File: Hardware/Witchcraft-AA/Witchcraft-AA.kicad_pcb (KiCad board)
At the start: 2 copper layers, 180 x 81 mm, 20 parts, among them J0 USB_C_Molex_201267-0005, J1 USB_C_Molex_201267-0005, J2 TE_2129567-1, U1 Z1 extreme, U2 LM26420-Q1xx-xxxx

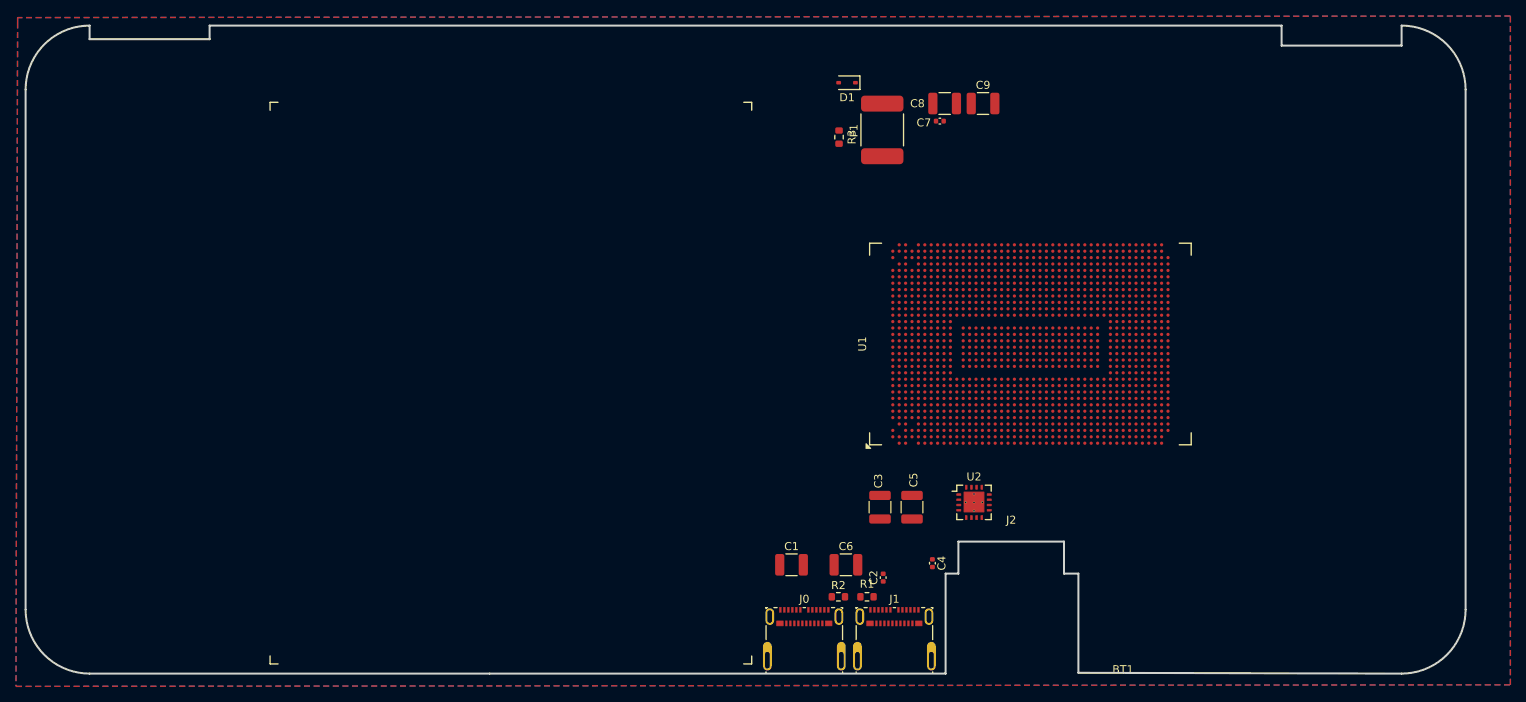
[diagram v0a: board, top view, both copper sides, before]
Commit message: Some chances to start/rectangle-buttons in mech, and startedmaking the M.2 ports.
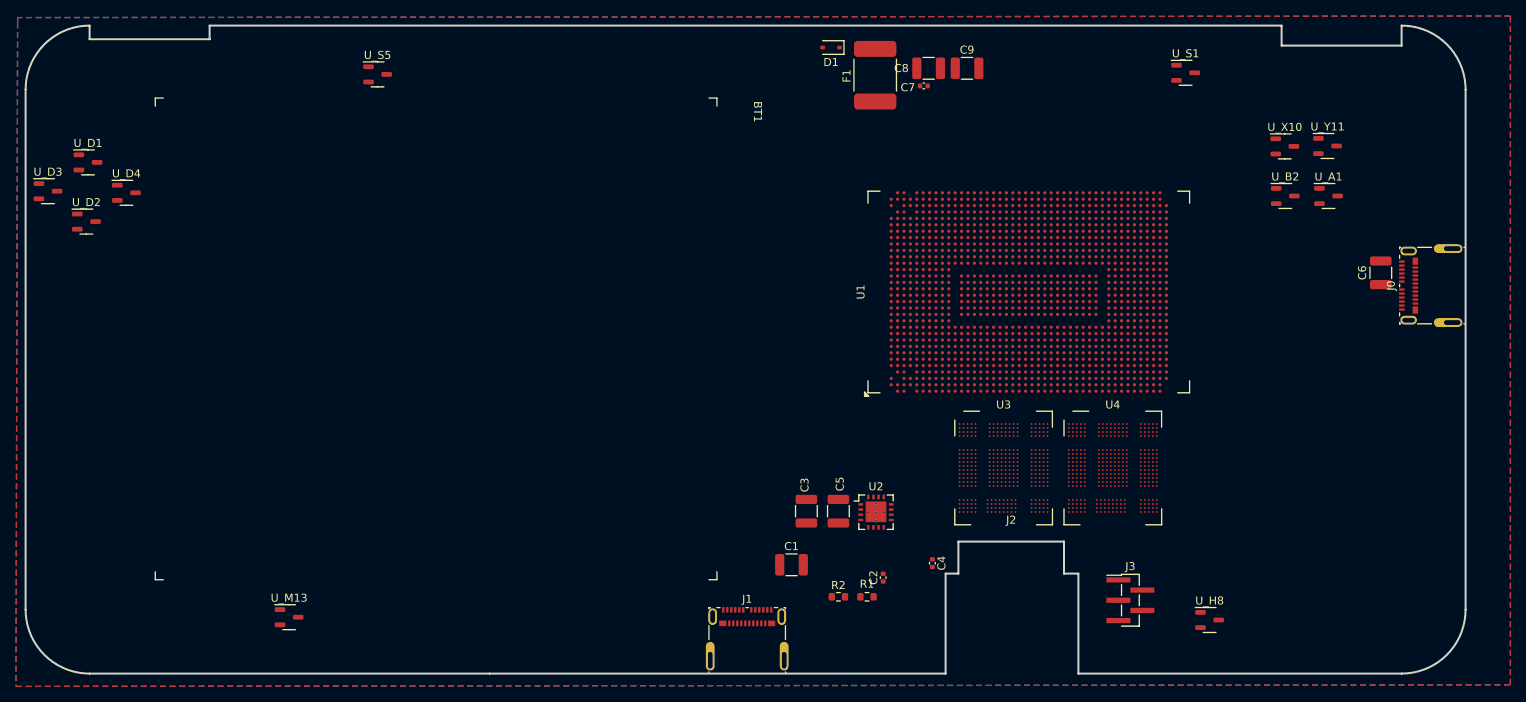
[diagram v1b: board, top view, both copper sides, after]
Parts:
- removed R3: R_ERJ-3GEYJ105V, Resistor_SMD:R_0603_1608Metric
- added J3: Conn_01x05_Socket, Connector_PinHeader_1.27mm:PinHeader_1x05_P1.27mm_Vertical_SMD_Pin1Left, F.Cu at (48.1, 31.3)
- added U3: K3LKCKC0BM, LRJ:SAMSUNG_FBGA-315_12x14mm_Layout23x23_P0.5mmP0.65mm, F.Cu at (32.2, 14.8)
- added U4: K3LKCKC0BM, LRJ:SAMSUNG_FBGA-315_12x14mm_Layout23x23_P0.5mmP0.65mm, F.Cu at (45.9, 14.8)
- added U_A1: Hall_Sensor, Package_TO_SOT_SMD:SOT-23-3, F.Cu at (72.9, -19.2)
- added U_B2: Hall_Sensor, Package_TO_SOT_SMD:SOT-23-3, F.Cu at (67.5, -19.2)
- added U_D1: Hall_Sensor, Package_TO_SOT_SMD:SOT-23-3, F.Cu at (-82.2, -23.4)
- added U_D2: Hall_Sensor, Package_TO_SOT_SMD:SOT-23-3, F.Cu at (-82.4, -16.0)
- added U_D3: Hall_Sensor, Package_TO_SOT_SMD:SOT-23-3, F.Cu at (-87.2, -19.8)
- added U_D4: Hall_Sensor, Package_TO_SOT_SMD:SOT-23-3, F.Cu at (-77.4, -19.6)
- added U_H8: Hall_Sensor, Package_TO_SOT_SMD:SOT-23-3, F.Cu at (58.0, 33.8)
- added U_M13: Hall_Sensor, Package_TO_SOT_SMD:SOT-23-3, F.Cu at (-57.1, 33.5)
- added U_S1: Hall_Sensor, Package_TO_SOT_SMD:SOT-23-3, F.Cu at (55.0, -34.6)
- added U_S5: Hall_Sensor, Package_TO_SOT_SMD:SOT-23-3, F.Cu at (-46.0, -34.4)
- added U_X10: Hall_Sensor, Package_TO_SOT_SMD:SOT-23-3, F.Cu at (67.4, -25.4)
- added U_Y11: Hall_Sensor, Package_TO_SOT_SMD:SOT-23-3, F.Cu at (72.7, -25.4)
- moved J0 90.4 mm to (86.0, -8.00), turned to 90 degrees
- moved C6 76.2 mm to (79.4, -9.60), turned to 90 degrees
- moved J1 18.4 mm to (0.20, 36.5)
- moved U2 12.3 mm to (16.3, 20.3)
- moved BT1 10.9 mm to (-38.7, -1.34), turned to -90 degrees
- moved C3 9.21 mm to (7.60, 20.2)
- moved C5 9.21 mm to (11.6, 20.2)
- moved F1 6.90 mm to (16.2, -34.2)
- moved U1 6.50 mm to (35.4, -7.20)
- moved C7 4.83 mm to (22.3, -33.0)
- moved D1 4.83 mm to (10.7, -37.8)
- moved C8 4.83 mm to (22.9, -35.2)
- moved C9 4.83 mm to (27.7, -35.2)
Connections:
- U2 pad 10: unconnected-(U2-SW2-Pad10) -> +1V8
- U2 pad 3: unconnected-(U2-SW1-Pad3) -> +3.3V
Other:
- outline, holes or cut-outs redrawn
